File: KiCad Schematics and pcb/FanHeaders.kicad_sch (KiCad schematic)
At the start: 11 parts, among them IC3 EMC2101-ACZL-TR, J4 Conn_01x02_Pin, M2 Fan_4pin, M3 Fan_4pin, M4 Fan_4pin, M5 Fan_4pin, Q1 DMN4035L-7, Q2 DMN4035L-7

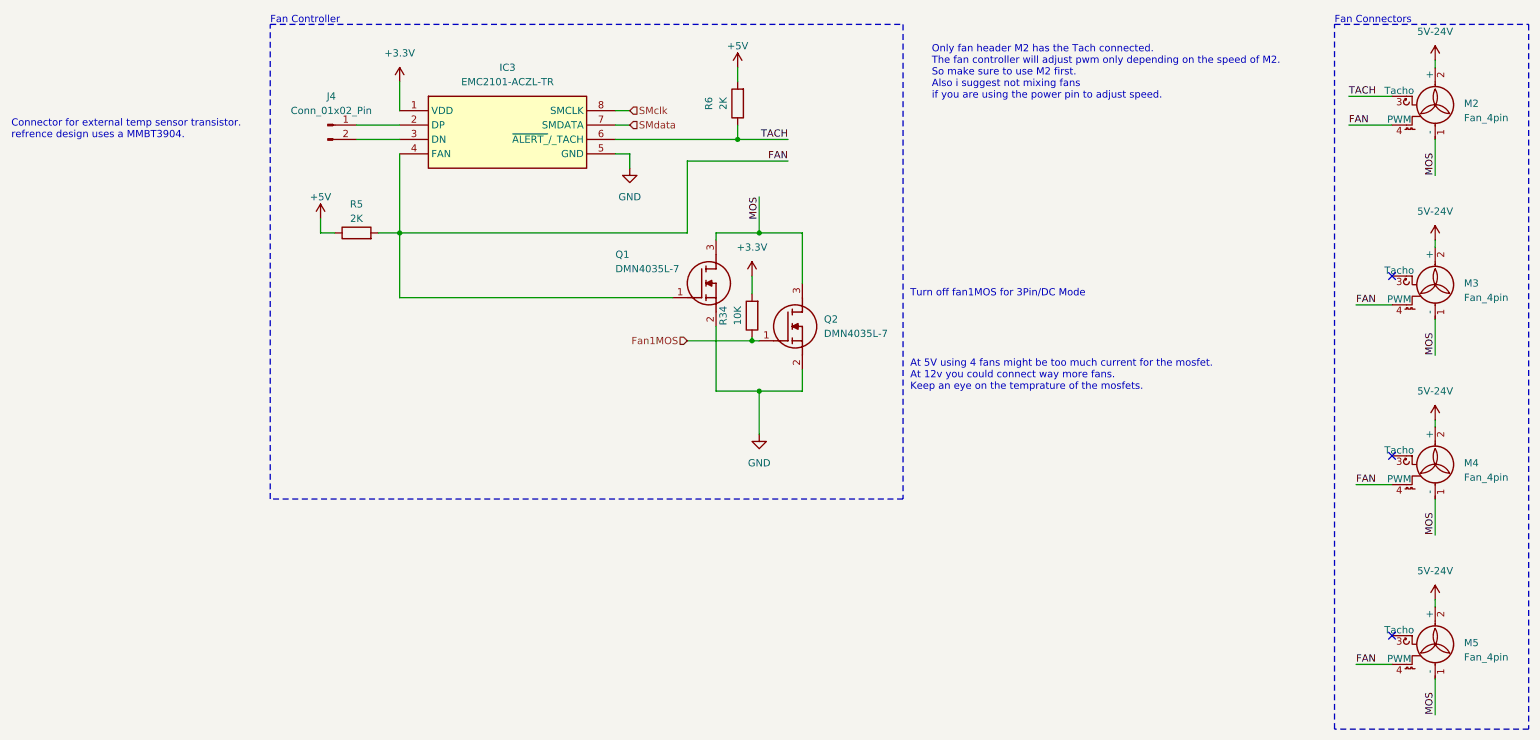
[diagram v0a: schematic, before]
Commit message: V0.2 wip
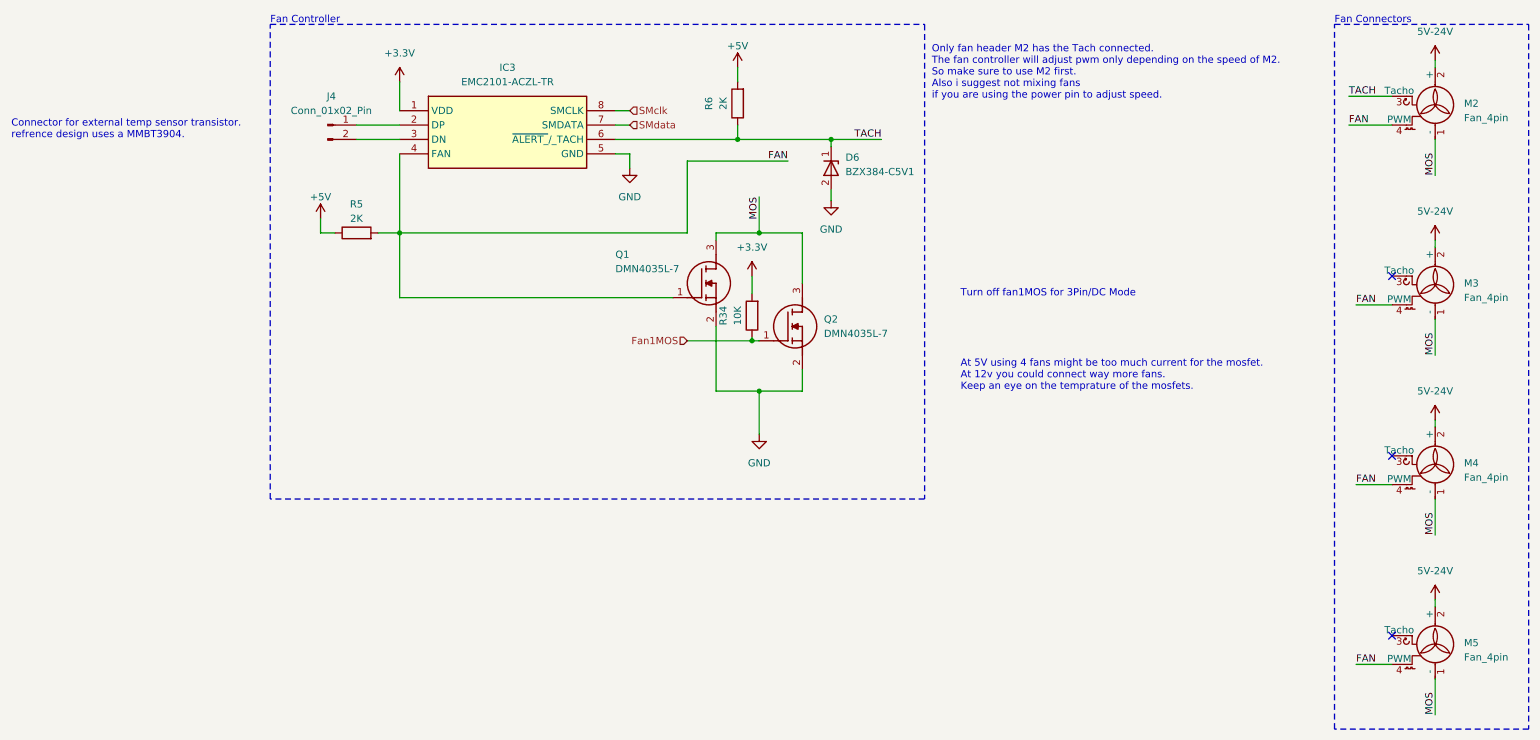
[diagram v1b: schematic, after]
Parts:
- added D6: BZX384-C5V1, ComponentSearch:SOD2512X110N, symbol ComponentSearch:BZX384-C5V1
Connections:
- net GND: now also D6.2 (A)
- net TACH: now also D6.1 (K)
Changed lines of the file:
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@@
     (title "ESPHome All in One Dev kit")
+  )
+  (junction (at 158.75 39.37) (diameter 0) (color 0 0 0 0)
   )
   (junction (at 144.78 74.93) (diameter 0) (color 0 0 0 0)
@@
     (stroke (width 0) (type default))
   )
+  (wire (pts (xy 158.75 48.26) (xy 158.75 50.165))
+    (stroke (width 0) (type default))
+  )
+  (wire (pts (xy 158.75 39.37) (xy 158.75 40.64))
+    (stroke (width 0) (type default))
+  )
   (wire (pts (xy 82.55 41.91) (xy 82.55 55.88))
     (stroke (width 0) (type default))
@@
     (stroke (width 0) (type default))
   )
+  (wire (pts (xy 158.75 39.37) (xy 167.64 39.37))
+    (stroke (width 0) (type default))
+  )
   (wire (pts (xy 250.19 36.83) (xy 257.81 36.83))
     (stroke (width 0) (type default))
@@
     (stroke (width 0) (type default))
   )
-  (wire (pts (xy 142.24 39.37) (xy 151.13 39.37))
+  (wire (pts (xy 142.24 39.37) (xy 158.75 39.37))
     (stroke (width 0) (type default))
   )
@@
     (fill (type none))
   )
-  (rectangle (start 59.69 19.05) (end 171.45 102.87)
+  (rectangle (start 59.69 19.05) (end 175.26 102.87)
     (stroke (width 0) (type dash))
     (fill (type none))
@@
   )
   (text "At 5V using 4 fans might be too much current for the mosfet.\nAt 12v you could connect way more fans.\nKeep an eye on the temprature of the mosfets."
-    (at 172.72 83.82 0)
+    (at 181.61 83.82 0)
     (effects (font (size 1.27 1.27)) (justify left bottom))
   )
@@
     (effects (font (size 1.27 1.27)) (justify left bottom))
   )
-  (text "Turn off fan1MOS for 3Pin/DC Mode" (at 172.72 67.31 0)
+  (text "Turn off fan1MOS for 3Pin/DC Mode" (at 181.61 67.31 0)
     (effects (font (size 1.27 1.27)) (justify left bottom))
   )
@@
     (effects (font (size 1.27 1.27)) (justify left bottom))
   )
-  (label "TACH" (at 151.13 39.37 180) (fields_autoplaced)
+  (label "TACH" (at 167.64 39.37 180) (fields_autoplaced)
     (effects (font (size 1.27 1.27)) (justify right bottom))
   )
@@
     )
   )
+  (symbol (lib_id "ComponentSearch:BZX384-C5V1") (at 159.385 36.195 270) (unit 1)
+    (in_bom yes) (on_board yes) (dnp no)
+    (property "Reference" "D6" (at 161.29 42.545 90)
+      (effects (font (size 1.27 1.27)) (justify left))
+    )
+    (property "Value" "BZX384-C5V1" (at 161.29 45.085 90)
+      (effects (font (size 1.27 1.27)) (justify left))
+    )
+    (property "Footprint" "ComponentSearch:SOD2512X110N" (at 61.925 47.625 0)
+      (effects (font (size 1.27 1.27)) (justify left top) hide)
+    )
+    (property "Datasheet" "https://datasheet.datasheetarchive.com/originals/distributors/Datasheets-20/DSA-380037.pdf" (at -38.075 47.625 0)
+      (effects (font (size 1.27 1.27)) (justify left top) hide)
+    )
+    (property "Height" "1.1" (at -238.075 47.625 0)
+      (effects (font (size 1.27 1.27)) (justify left top) hide)
+    )
+    (property "Manufacturer_Name" "Nexperia" (at -338.075 47.625 0)
+      (effects (font (size 1.27 1.27)) (justify left top) hide)
+    )
+    (property "Manufacturer_Part_Number" "BZX384-C5V1" (at -438.075 47.625 0)
+      (effects (font (size 1.27 1.27)) (justify left top) hide)
+    )
+    (property "Mouser Part Number" "N/A" (at -538.075 47.625 0)
+      (effects (font (size 1.27 1.27)) (justify left top) hide)
+    )
+    (property "Mouser Price/Stock" "https://www.mouser.co.uk/ProductDetail/Nexperia/BZX384-C5V1?qs=vHuUswq2%252Bszm012Dq%252BI0lA%3D%3D" (at -638.075 47.625 0)
+      (effects (font (size 1.27 1.27)) (justify left top) hide)
+    )
+    (property "Arrow Part Number" "" (at -738.075 47.625 0)
+      (effects (font (size 1.27 1.27)) (justify left top) hide)
+    )
+    (property "Arrow Price/Stock" "" (at -838.075 47.625 0)
+      (effects (font (size 1.27 1.27)) (justify left top) hide)
+    )
+    (pin "1")
+    (pin "2")
+    (instances
+      (project "ESPHome AIO"
+        (path "/5cdf3b4f-d143-42e3-ac6f-eec5265de1fa/de469bc3-ee25-4a6a-9df7-c0a954ea29b4"
+          (reference "D6") (unit 1)
+        )
+      )
+    )
+  )
   (symbol (lib_id "ComponentSearch:DMN4035L-7") (at 146.05 74.93 0) (unit 1)
     (in_bom yes) (on_board yes) (dnp no) (fields_autoplaced)
@@
         )
       )
+    )
+  )
+  (symbol (lib_id "power:GND") (at 158.75 50.165 0) (unit 1)
+    (in_bom yes) (on_board yes) (dnp no) (fields_autoplaced)
+    (property "Reference" "#PWR072" (at 158.75 56.515 0)
+      (effects (font (size 1.27 1.27)) hide)
+    )
+    (property "Value" "GND" (at 158.75 55.245 0)
+      (effects (font (size 1.27 1.27)))
+    )
+    (property "Footprint" "" (at 158.75 50.165 0)
+      (effects (font (size 1.27 1.27)) hide)
+    )
+    (property "Datasheet" "" (at 158.75 50.165 0)
+      (effects (font (size 1.27 1.27)) hide)
+    )
+    (pin "1")
+    (instances
+      (project "ESPHome AIO"
+        (path "/5cdf3b4f-d143-42e3-ac6f-eec5265de1fa/de469bc3-ee25-4a6a-9df7-c0a954ea29b4"
+          (reference "#PWR072") (unit 1)
+        )
+      )
